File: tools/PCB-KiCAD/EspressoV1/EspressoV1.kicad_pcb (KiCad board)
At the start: 2 copper layers, 92.7 x 72.4 mm, 29 parts, among them J1 Relay_Board

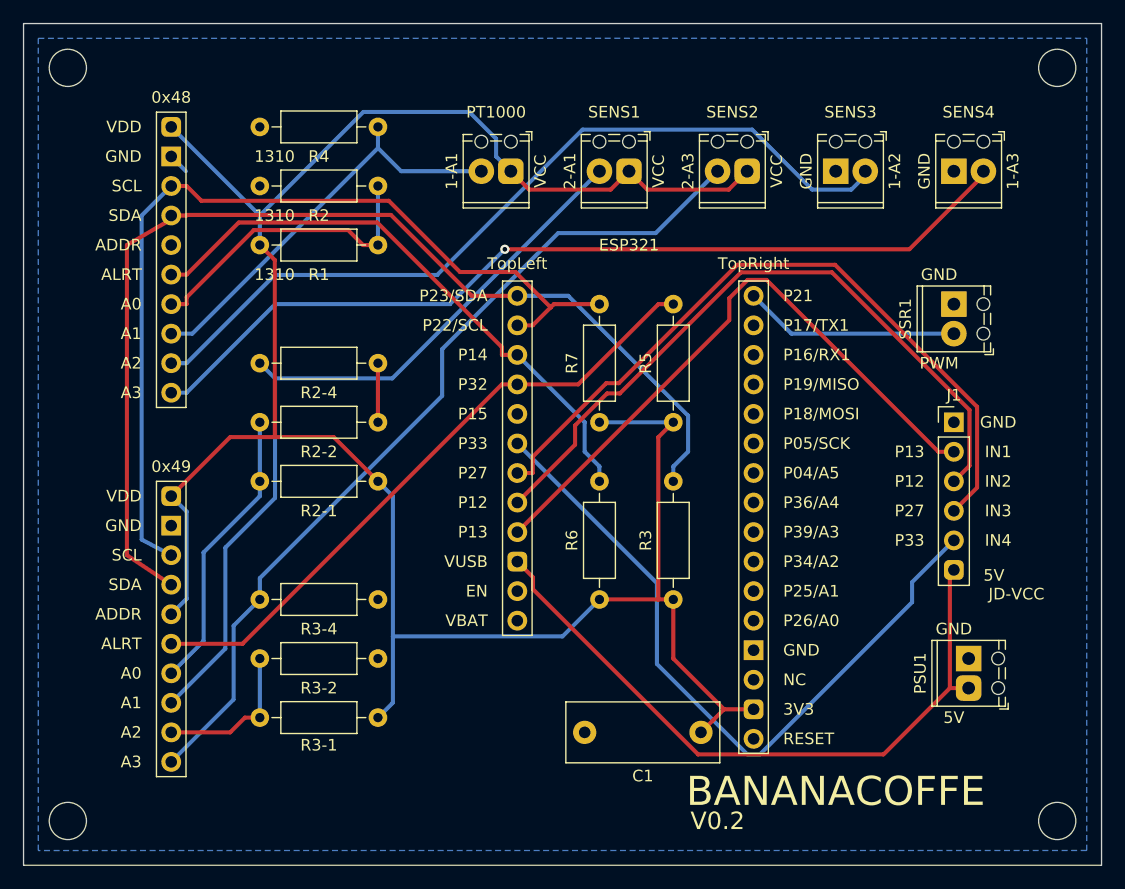
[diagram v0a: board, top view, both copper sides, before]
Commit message: PCB V2
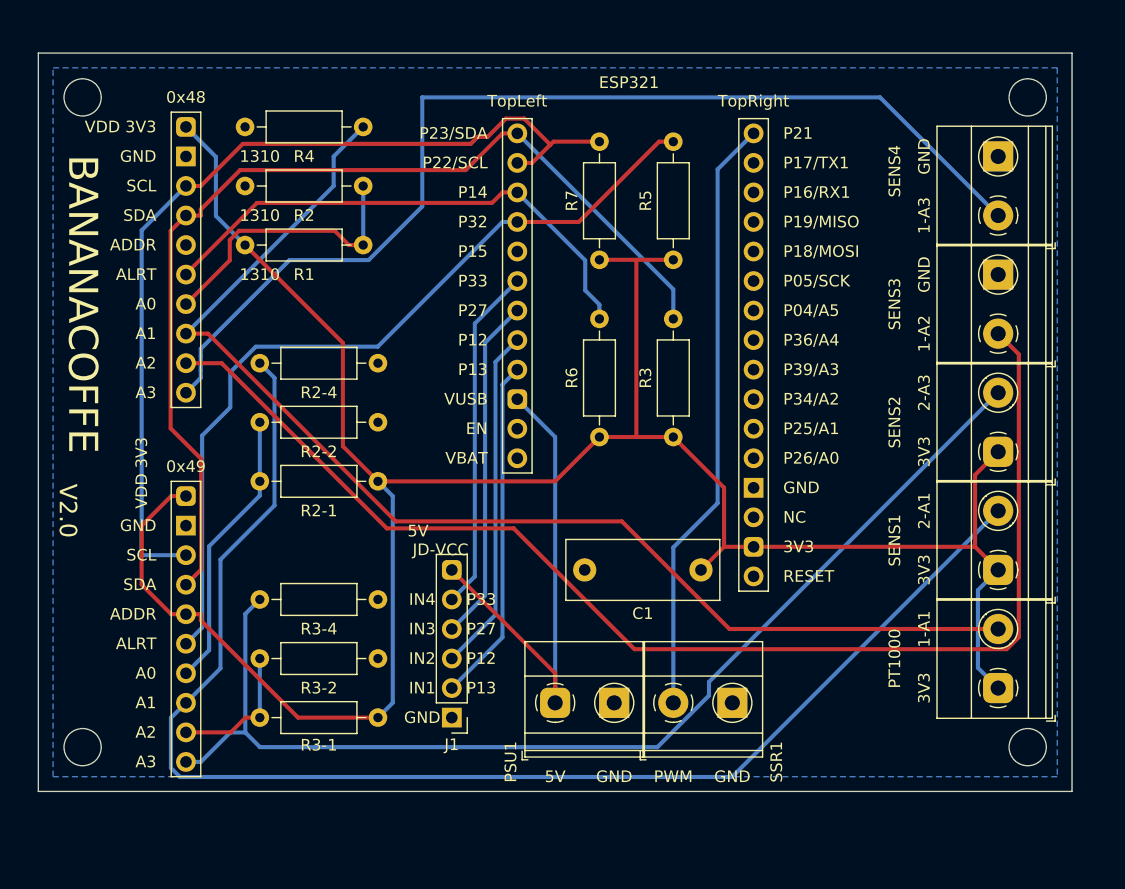
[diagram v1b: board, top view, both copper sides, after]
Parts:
- PSU1, PT1000, SENS1, SENS2, SENS3, SENS4, SSR1: footprint TerminalBlock_Phoenix:TerminalBlock_Phoenix_MPT-0,5-2-2.54_1x02_P2.54mm_Horizontal -> TerminalBlock_Phoenix:TerminalBlock_Phoenix_MKDS-1,5-2-5.08_1x02_P5.08mm_Horizontal
- moved PT1000 61.1 mm to (177.8, 108.0), turned to 90 degrees
- moved J1 50.1 mm to (130.8, 110.5), turned to 180 degrees
- moved SENS1 46.7 mm to (177.8, 97.8), turned to 90 degrees
- moved SSR1 39.9 mm to (149.9, 109.2), turned to 0 degrees
- moved PSU1 35.6 mm to (139.7, 109.2), turned to 0 degrees
- moved SENS2 32.4 mm to (177.8, 87.6), turned to 90 degrees
- moved SENS3 18.1 mm to (177.8, 77.5), turned to 90 degrees
- moved C1 14.0 mm to (152.2, 97.8)
- moved ESP321 14.0 mm to (146.6, 71.7)
- moved R3 14.0 mm to (149.9, 86.4)
- moved R5 14.0 mm to (149.9, 71.1)
- moved R6 14.0 mm to (143.5, 86.4)
- moved R7 14.0 mm to (143.5, 71.1)
- moved UR 6.84 mm to (180.3, 113.0)
- moved UL 6.48 mm to (99.1, 113.0)
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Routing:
- net Net-(0x48-Pad5): track 35.9 -> 104.5 mm
- net Net-(0x49-Pad5): track 68.7 -> 120.0 mm
- net Net-(0x48-Pad6): track 71.0 -> 109.1 mm
- net Net-(ESP321-PadP21): track 18.6 -> 51.8 mm
- net Net-(ESP321-PadP27): track 62.6 -> 29.7 mm
- net Net-(ESP321-PadP33): track 61.3 -> 29.7 mm
- net Net-(ESP321-PadP12): track 59.7 -> 29.7 mm
- net Net-(ESP321-PadP13): track 53.8 -> 29.7 mm
- net Net-(0x49-Pad7): track 75.2 -> 96.7 mm
- net Net-(ESP321-PadVUSB): track 59.0 -> 42.6 mm
- net Net-(0x49-Pad2): track 55.3 -> 71.2 mm
- net Net-(0x48-Pad7): track 77.9 -> 91.5 mm, vias 1 -> 0
- net Net-(0x48-Pad9): track 94.1 -> 87.2 mm
- net GND: track 6.88 -> 0.00 mm
- net Net-(0x48-Pad2): track 50.5 -> 45.3 mm
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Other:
- board size 92.7 x 72.4 mm -> 88.9 x 63.5 mm
- board text added: "3V3"
- board text added: "V2.0"
- board text removed: "V0.2"
- board text removed: "VCC"
